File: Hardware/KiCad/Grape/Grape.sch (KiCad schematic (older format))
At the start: 0 parts

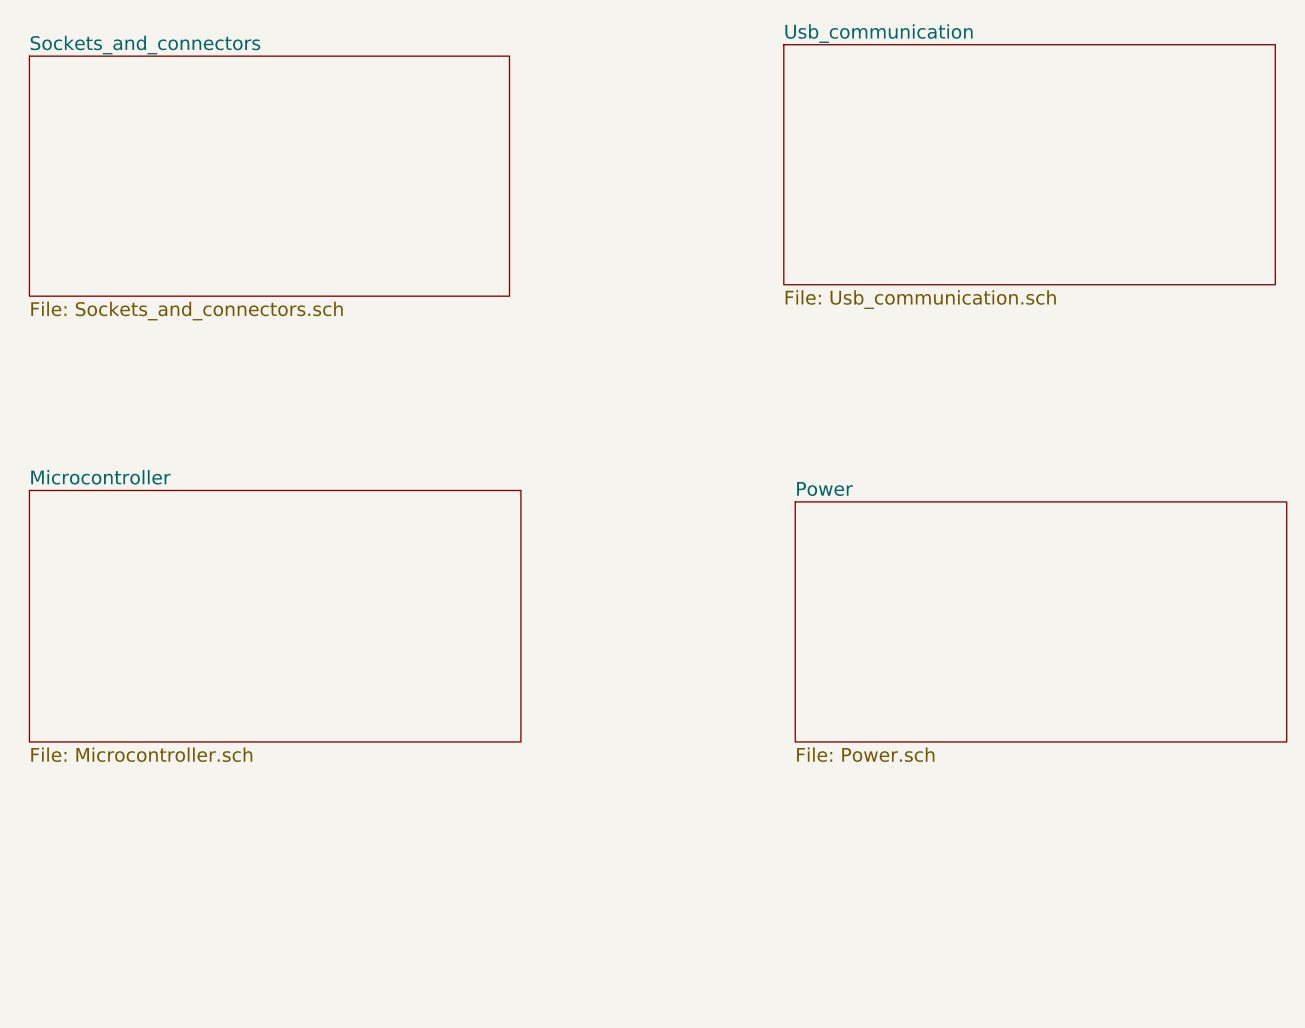
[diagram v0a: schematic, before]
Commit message: Esquema terminado y  ERC pasado
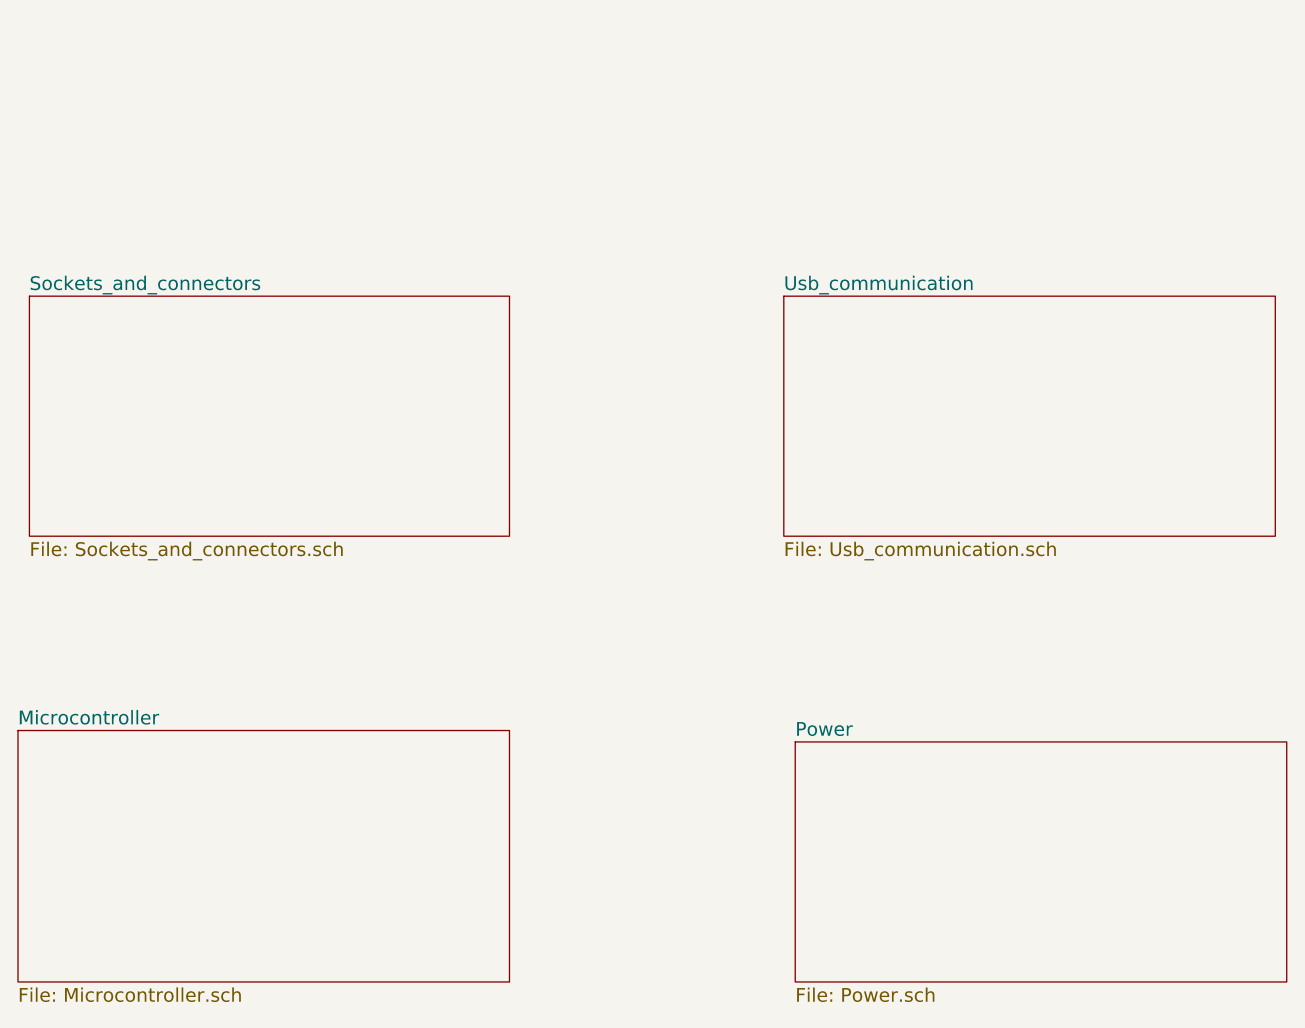
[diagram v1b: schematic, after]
